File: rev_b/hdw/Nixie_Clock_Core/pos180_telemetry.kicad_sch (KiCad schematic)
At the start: 25 parts, among them Q701 BSS192PH6327FTSA1, U701 OPA333xxDCK, U704 OPA333xxDCK, U705 OPA333xxDCK

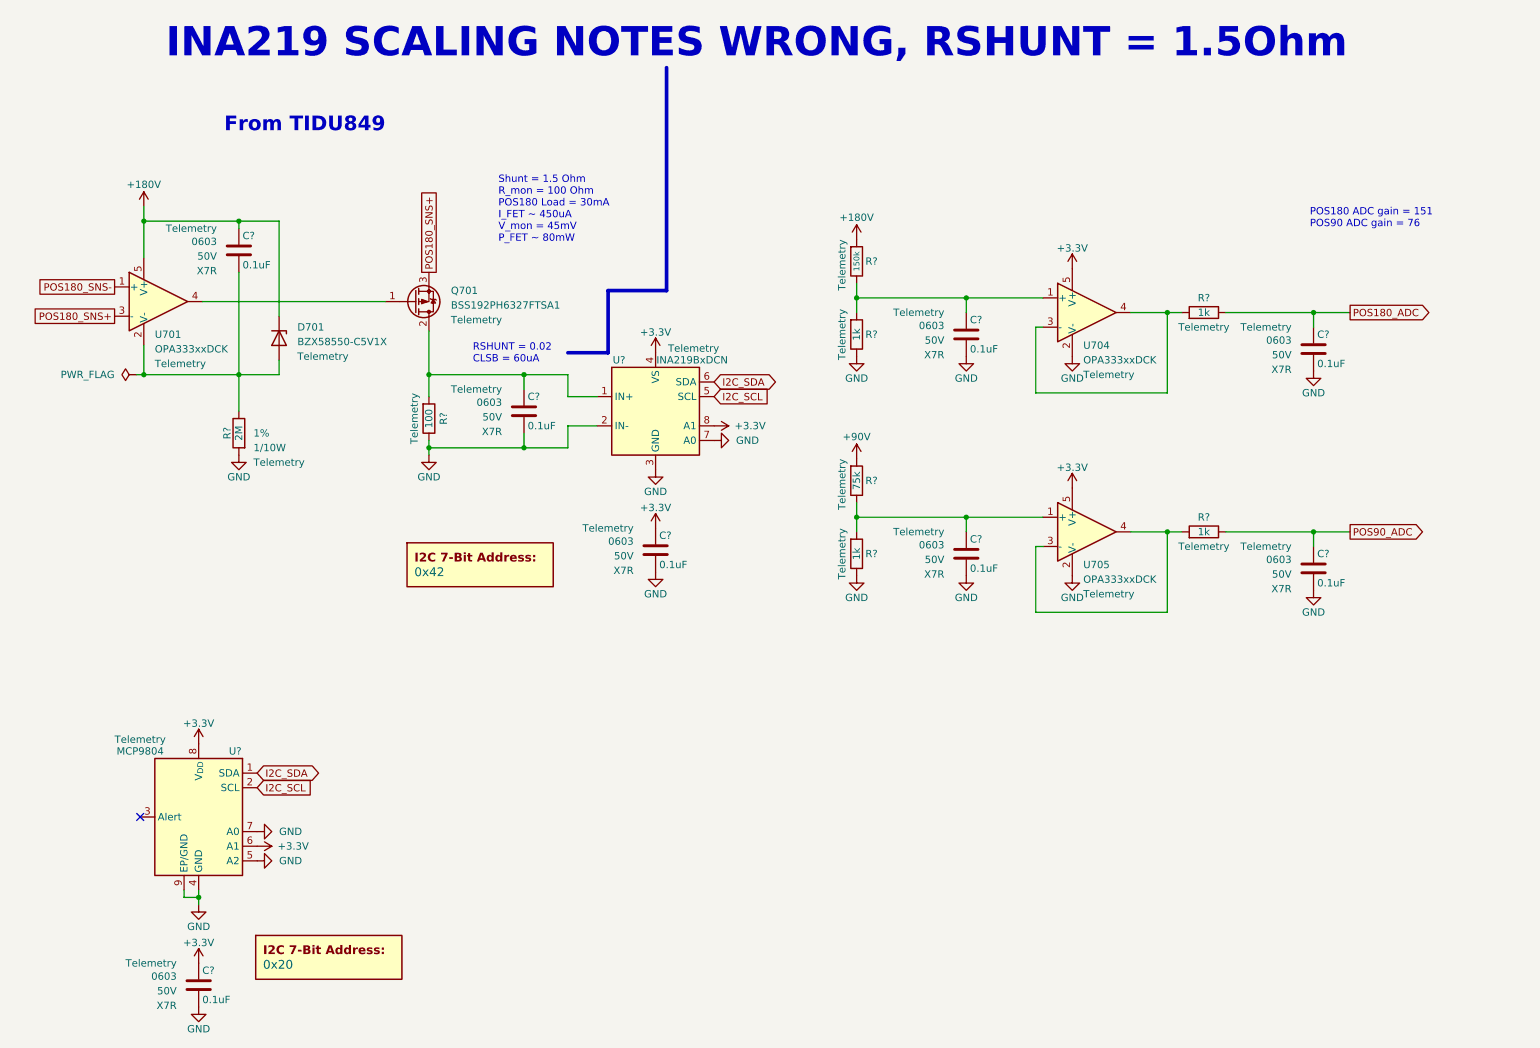
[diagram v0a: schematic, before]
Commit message: lots more PCB placement
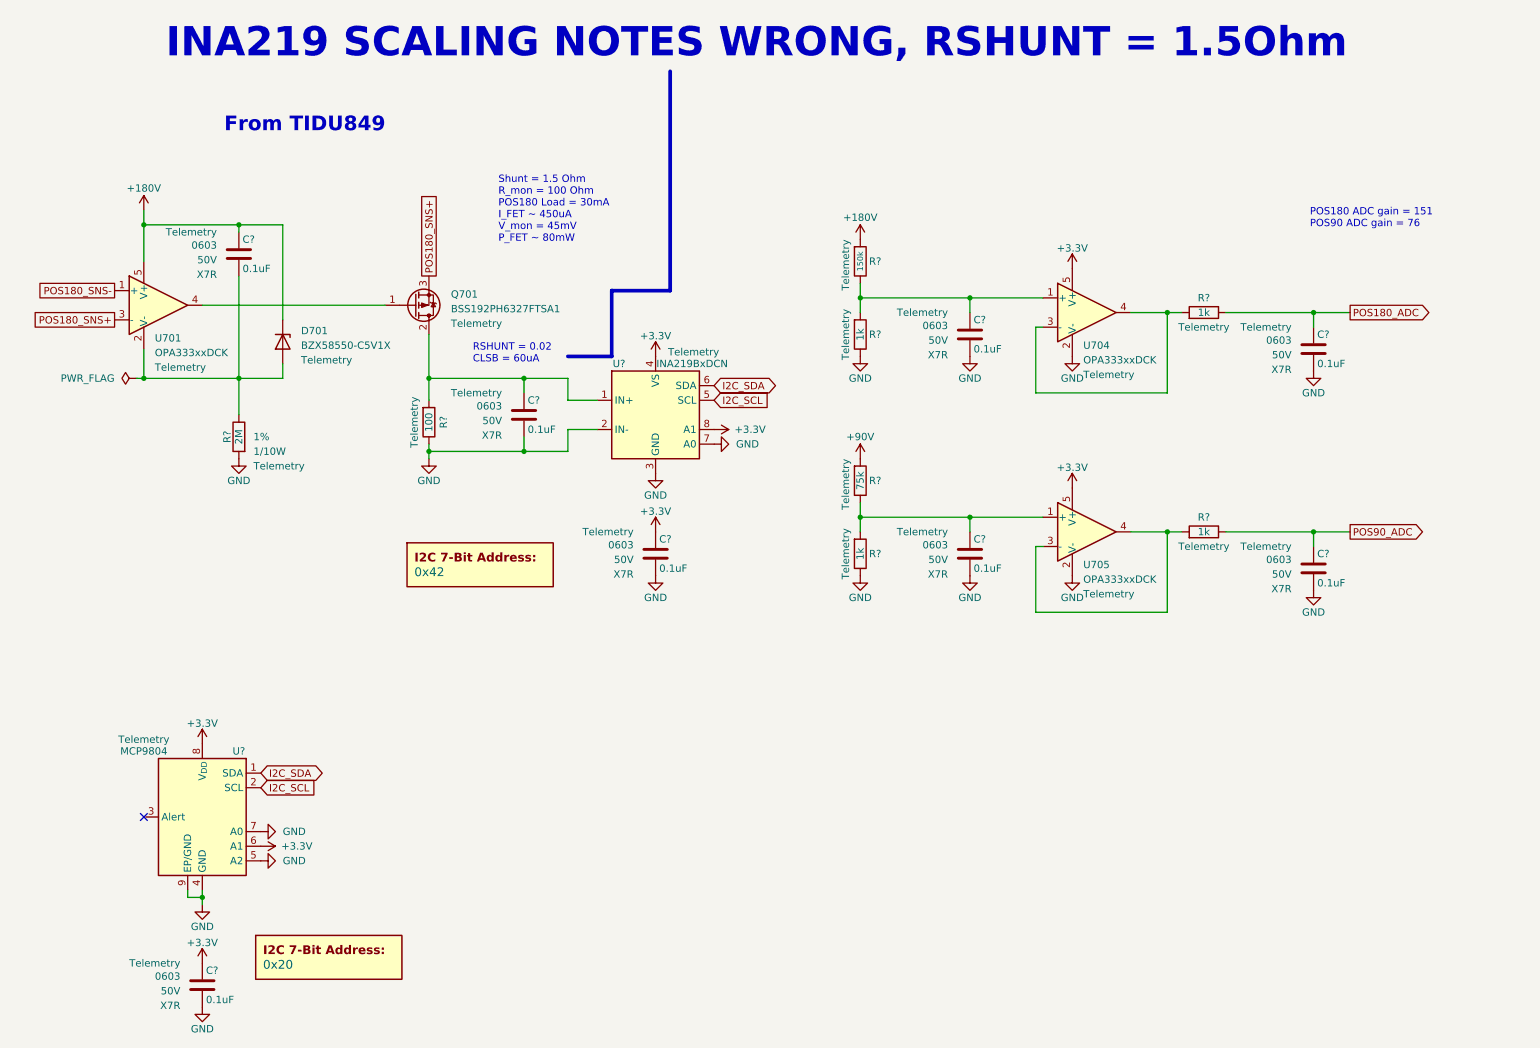
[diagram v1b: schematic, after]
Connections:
- net +180V: no longer R?.1
- new net +90V: R?.1
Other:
- moved on the sheet: C?, D701, Q701, R?, U701, U?
